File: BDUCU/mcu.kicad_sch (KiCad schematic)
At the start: 15 parts, among them SW1 SW_Push, U8 ATmega328-A, Y1 20MHz

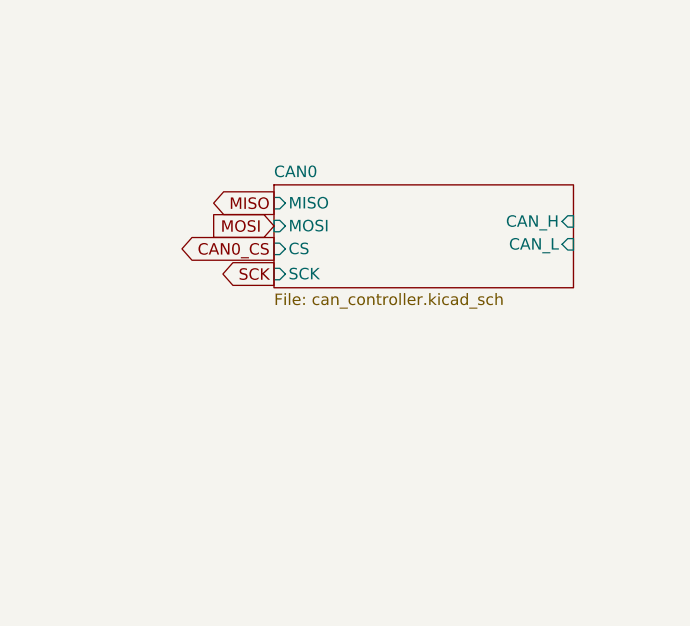
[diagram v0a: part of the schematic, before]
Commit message: BDUCU did stuffs
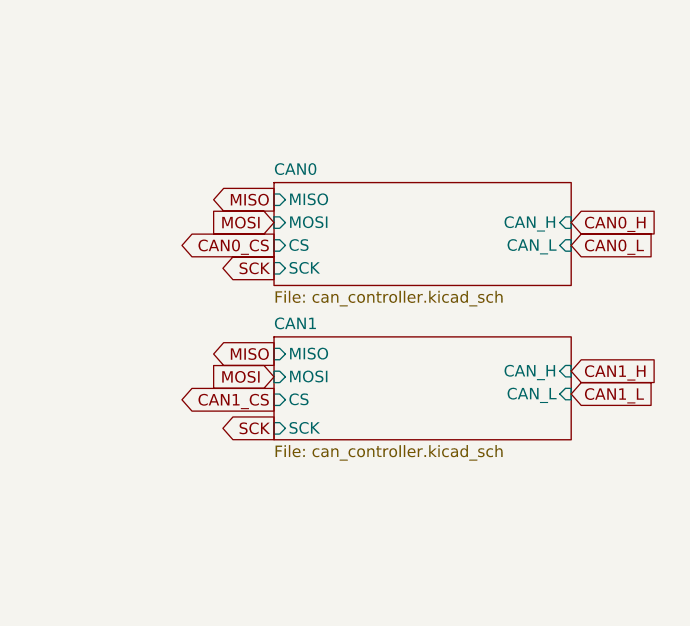
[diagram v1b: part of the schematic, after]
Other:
- added sheet CAN1 (can_controller.kicad_sch)
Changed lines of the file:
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@@
     )
   )
-  (global_label "CAN0_CS" (shape output) (at 209.55 46.736 180) (fields_autoplaced)
-    (effects (font (size 1.27 1.27)) (justify right))
-    (property "Intersheetrefs" "${INTERSHEET_REFS}" (at 198.2191 46.736 0)
+  (global_label "CAN0_CS" (shape output) (at 209.55 46.355 180) (fields_autoplaced)
+    (effects (font (size 1.27 1.27)) (justify right))
+    (property "Intersheetrefs" "${INTERSHEET_REFS}" (at 198.2191 46.355 0)
       (effects (font (size 1.27 1.27)) (justify right) hide)
     )
@@
     )
   )
+  (global_label "CAN0_H" (shape input) (at 242.57 43.815 0) (fields_autoplaced)
+    (effects (font (size 1.27 1.27)) (justify left))
+    (property "Intersheetrefs" "${INTERSHEET_REFS}" (at 252.7519 43.815 0)
+      (effects (font (size 1.27 1.27)) (justify left) hide)
+    )
+  )
+  (global_label "SCK" (shape output) (at 209.55 66.675 180) (fields_autoplaced)
+    (effects (font (size 1.27 1.27)) (justify right))
+    (property "Intersheetrefs" "${INTERSHEET_REFS}" (at 202.8153 66.675 0)
+      (effects (font (size 1.27 1.27)) (justify right) hide)
+    )
+  )
   (global_label "TS_ACT_5" (shape input) (at 71.374 104.648 0) (fields_autoplaced)
     (effects (font (size 1.27 1.27)) (justify left))
@@
     )
   )
+  (global_label "CAN1_CS" (shape output) (at 209.55 63.5 180) (fields_autoplaced)
+    (effects (font (size 1.27 1.27)) (justify right))
+    (property "Intersheetrefs" "${INTERSHEET_REFS}" (at 198.2191 63.5 0)
+      (effects (font (size 1.27 1.27)) (justify right) hide)
+    )
+  )
   (global_label "RST" (shape input) (at 114.935 117.475 180) (fields_autoplaced)
     (effects (font (size 1.27 1.27)) (justify right))
@@
     )
   )
+  (global_label "MOSI" (shape input) (at 209.55 60.96 180) (fields_autoplaced)
+    (effects (font (size 1.27 1.27)) (justify right))
+    (property "Intersheetrefs" "${INTERSHEET_REFS}" (at 202.048 60.96 0)
+      (effects (font (size 1.27 1.27)) (justify right) hide)
+    )
+  )
   (global_label "AIR+_5" (shape output) (at 71.374 94.488 0) (fields_autoplaced)
     (effects (font (size 1.27 1.27)) (justify left))
@@
     )
   )
+  (global_label "MISO" (shape output) (at 209.55 58.42 180) (fields_autoplaced)
+    (effects (font (size 1.27 1.27)) (justify right))
+    (property "Intersheetrefs" "${INTERSHEET_REFS}" (at 201.9686 58.42 0)
+      (effects (font (size 1.27 1.27)) (justify right) hide)
+    )
+  )
   (global_label "HALL_HI" (shape input) (at 71.374 79.248 0) (fields_autoplaced)
     (effects (font (size 1.27 1.27)) (justify left))
@@
     )
   )
+  (global_label "CAN1_H" (shape input) (at 242.57 60.325 0) (fields_autoplaced)
+    (effects (font (size 1.27 1.27)) (justify left))
+    (property "Intersheetrefs" "${INTERSHEET_REFS}" (at 252.7519 60.325 0)
+      (effects (font (size 1.27 1.27)) (justify left) hide)
+    )
+  )
   (global_label "MOSI" (shape input) (at 71.374 56.388 0) (fields_autoplaced)
     (effects (font (size 1.27 1.27)) (justify left))
@@
     )
   )
-  (global_label "MOSI" (shape input) (at 209.55 44.196 180) (fields_autoplaced)
-    (effects (font (size 1.27 1.27)) (justify right))
-    (property "Intersheetrefs" "${INTERSHEET_REFS}" (at 202.048 44.196 0)
+  (global_label "MOSI" (shape input) (at 209.55 43.815 180) (fields_autoplaced)
+    (effects (font (size 1.27 1.27)) (justify right))
+    (property "Intersheetrefs" "${INTERSHEET_REFS}" (at 202.048 43.815 0)
       (effects (font (size 1.27 1.27)) (justify right) hide)
     )
@@
     )
   )
+  (global_label "CAN0_L" (shape input) (at 242.57 46.355 0) (fields_autoplaced)
+    (effects (font (size 1.27 1.27)) (justify left))
+    (property "Intersheetrefs" "${INTERSHEET_REFS}" (at 252.4495 46.355 0)
+      (effects (font (size 1.27 1.27)) (justify left) hide)
+    )
+  )
   (global_label "CAN0_CS" (shape output) (at 71.374 53.848 0) (fields_autoplaced)
     (effects (font (size 1.27 1.27)) (justify left))
@@
     )
   )
-  (global_label "SCK" (shape output) (at 209.55 49.53 180) (fields_autoplaced)
-    (effects (font (size 1.27 1.27)) (justify right))
-    (property "Intersheetrefs" "${INTERSHEET_REFS}" (at 202.8153 49.53 0)
-      (effects (font (size 1.27 1.27)) (justify right) hide)
-    )
-  )
-  (global_label "MISO" (shape output) (at 209.55 41.656 180) (fields_autoplaced)
-    (effects (font (size 1.27 1.27)) (justify right))
-    (property "Intersheetrefs" "${INTERSHEET_REFS}" (at 201.9686 41.656 0)
+  (global_label "SCK" (shape output) (at 209.55 48.895 180) (fields_autoplaced)
+    (effects (font (size 1.27 1.27)) (justify right))
+    (property "Intersheetrefs" "${INTERSHEET_REFS}" (at 202.8153 48.895 0)
+      (effects (font (size 1.27 1.27)) (justify right) hide)
+    )
+  )
+  (global_label "CAN1_L" (shape input) (at 242.57 62.865 0) (fields_autoplaced)
+    (effects (font (size 1.27 1.27)) (justify left))
+    (property "Intersheetrefs" "${INTERSHEET_REFS}" (at 252.4495 62.865 0)
+      (effects (font (size 1.27 1.27)) (justify left) hide)
+    )
+  )
+  (global_label "MISO" (shape output) (at 209.55 41.275 180) (fields_autoplaced)
+    (effects (font (size 1.27 1.27)) (justify right))
+    (property "Intersheetrefs" "${INTERSHEET_REFS}" (at 201.9686 41.275 0)
       (effects (font (size 1.27 1.27)) (justify right) hide)
     )
@@
     )
   )
-  (sheet (at 209.55 39.624) (size 33.274 11.43) (fields_autoplaced)
+  (sheet (at 209.55 39.37) (size 33.02 11.43) (fields_autoplaced)
     (stroke (width 0.1524) (type solid))
     (fill (color 0 0 0 0.0000))
-    (property "Sheetname" "CAN0" (at 209.55 38.9124 0)
+    (property "Sheetname" "CAN0" (at 209.55 38.6584 0)
       (effects (font (size 1.27 1.27)) (justify left bottom))
     )
-    (property "Sheetfile" "can_controller.kicad_sch" (at 209.55 51.6386 0)
+    (property "Sheetfile" "can_controller.kicad_sch" (at 209.55 51.3846 0)
       (effects (font (size 1.27 1.27)) (justify left top))
     )
-    (pin "MISO" input (at 209.55 41.656 180)
+    (pin "MISO" input (at 209.55 41.275 180)
       (effects (font (size 1.27 1.27)) (justify left))
     )
-    (pin "MOSI" input (at 209.55 44.196 180)
+    (pin "MOSI" input (at 209.55 43.815 180)
       (effects (font (size 1.27 1.27)) (justify left))
     )
-    (pin "CS" input (at 209.55 46.736 180)
+    (pin "CS" input (at 209.55 46.355 180)
       (effects (font (size 1.27 1.27)) (justify left))
     )
-    (pin "SCK" input (at 209.55 49.53 180)
+    (pin "SCK" input (at 209.55 48.895 180)
       (effects (font (size 1.27 1.27)) (justify left))
     )
-    (pin "CAN_H" input (at 242.824 43.688 0)
-      (effects (font (size 1.27 1.27)) (justify right))
-    )
-    (pin "CAN_L" input (at 242.824 46.228 0)
+    (pin "CAN_H" input (at 242.57 43.815 0)
+      (effects (font (size 1.27 1.27)) (justify right))
+    )
+    (pin "CAN_L" input (at 242.57 46.355 0)
       (effects (font (size 1.27 1.27)) (justify right))
     )
@@
       )
     )
+  )
+  (sheet (at 209.55 56.515) (size 33.02 11.43) (fields_autoplaced)
+    (stroke (width 0.1524) (type solid))
+    (fill (color 0 0 0 0.0000))
+    (property "Sheetname" "CAN1" (at 209.55 55.8034 0)
+      (effects (font (size 1.27 1.27)) (justify left bottom))
+    )
+    (property "Sheetfile" "can_controller.kicad_sch" (at 209.55 68.5296 0)
+      (effects (font (size 1.27 1.27)) (justify left top))
+    )
+    (pin "MISO" input (at 209.55 58.42 180)
+      (effects (font (size 1.27 1.27)) (justify left))
+    )
+    (pin "MOSI" input (at 209.55 60.96 180)
+      (effects (font (size 1.27 1.27)) (justify left))
+    )
+    (pin "CS" input (at 209.55 63.5 180)
+      (effects (font (size 1.27 1.27)) (justify left))
+    )
+    (pin "SCK" input (at 209.55 66.675 180)
+      (effects (font (size 1.27 1.27)) (justify left))
+    )
+    (pin "CAN_H" input (at 242.57 60.325 0)
+      (effects (font (size 1.27 1.27)) (justify right))
+    )
+    (pin "CAN_L" input (at 242.57 62.865 0)
+      (effects (font (size 1.27 1.27)) (justify right))
+    )
+    (instances
+      (project "BDUCU"
+        (path "/9942a424-e19d-4ffb-8473-f960b5c811cf/8fc427df-2d97-44b9-b479-5014f2f05880" (page "12"))
+      )
+    )

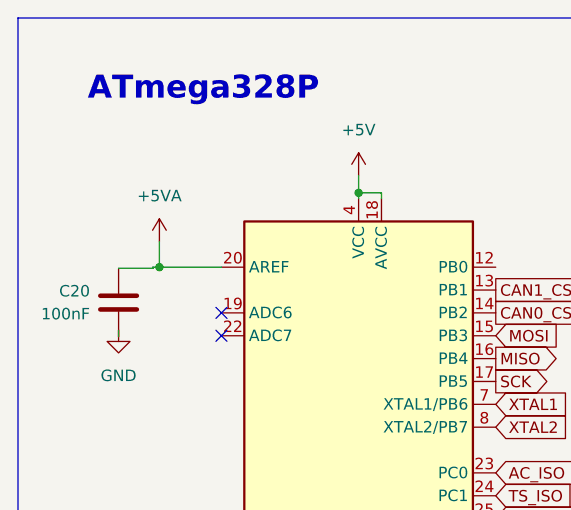
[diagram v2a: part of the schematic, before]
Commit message: BDUCU COMMIT
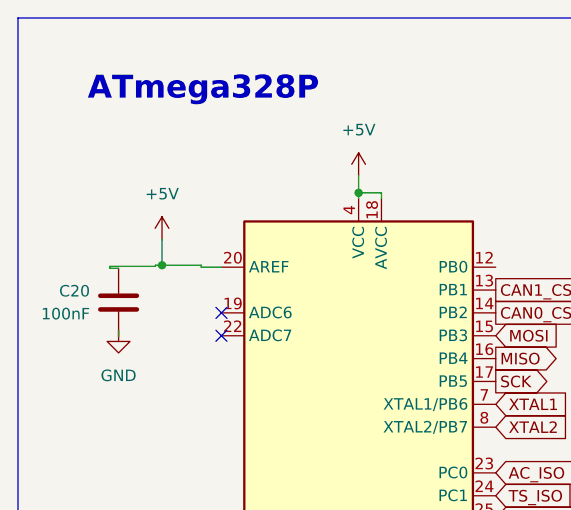
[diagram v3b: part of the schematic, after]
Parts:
- AVR-ISP1: footprint Connector_PinHeader_2.54mm:PinHeader_2x03_P2.54mm_Vertical -> Connector_PinHeader_2.54mm:PinHeader_2x03_P2.54mm_Vertical_SMD
- Y1: value 20MHz -> 16MHz
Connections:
- net +5VA is gone; now on net +5V: C20.2, U8.20 (AREF)
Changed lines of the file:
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@@
 	)
 	(junction
-		(at 34.001 48.768)
+		(at 34.29 48.5525)
 		(diameter 0)
 		(color 0 0 0 0)
@@
 	(wire
 		(pts
-			(xy 34.001 48.768) (xy 40.894 48.768)
+			(xy 28.483 48.6795) (xy 33.563 48.6795)
+		)
+		(stroke
+			(width 0)
+			(type default)
+		)
+	)
+	(wire
+		(pts
+			(xy 34.29 48.5525) (xy 38.643 48.5525)
 		)
 		(stroke
@@
 	(wire
 		(pts
-			(xy 34.001 45.9355) (xy 34.001 48.768)
+			(xy 34.29 45.72) (xy 34.29 48.5525)
+		)
+		(stroke
+			(width 0)
+			(type default)
+		)
+	)
+	(wire
+		(pts
+			(xy 28.483 48.895) (xy 29.464 48.895)
 		)
 		(stroke
@@
 	(wire
 		(pts
+			(xy 28.483 48.6795) (xy 28.483 48.895)
+		)
+		(stroke
+			(width 0)
+			(type default)
+		)
+	)
+	(wire
+		(pts
 			(xy 111.76 86.995) (xy 111.76 95.25)
 		)
@@
 	(wire
 		(pts
-			(xy 33.274 48.895) (xy 33.274 48.768)
+			(xy 33.563 48.6795) (xy 33.563 48.5525)
 		)
 		(stroke
@@
 	(wire
 		(pts
+			(xy 38.643 48.768) (xy 40.894 48.768)
+		)
+		(stroke
+			(width 0)
+			(type default)
+		)
+	)
+	(wire
+		(pts
 			(xy 100.965 41.275) (xy 100.965 40.64)
 		)
@@
 	(wire
 		(pts
+			(xy 38.643 48.5525) (xy 38.643 48.768)
+		)
+		(stroke
+			(width 0)
+			(type default)
+		)
+	)
+	(wire
+		(pts
 			(xy 125.73 86.995) (xy 125.73 95.25)
 		)
@@
 	(wire
 		(pts
-			(xy 33.274 48.768) (xy 34.001 48.768)
-		)
-		(stroke
-			(width 0)
-			(type default)
-		)
-	)
-	(wire
-		(pts
-			(xy 29.464 48.895) (xy 33.274 48.895)
+			(xy 33.563 48.5525) (xy 34.29 48.5525)
 		)
 		(stroke
@@
 				(path "/9942a424-e19d-4ffb-8473-f960b5c811cf/8fc427df-2d97-44b9-b479-5014f2f05880"
 					(reference "D3")
+					(unit 1)
+				)
+			)
+		)
+	)
+	(symbol
+		(lib_id "power:+5V")
+		(at 34.29 45.72 0)
+		(unit 1)
+		(exclude_from_sim no)
+		(in_bom yes)
+		(on_board yes)
+		(dnp no)
+		(fields_autoplaced yes)
+		(property "Reference" "#PWR033"
+			(at 34.29 49.53 0)
+			(effects
+				(font
+					(size 1.27 1.27)
+				)
+				(hide yes)
+			)
+		)
+		(property "Value" "+5V"
+			(at 34.29 40.64 0)
+			(effects
+				(font
+					(size 1.27 1.27)
+				)
+			)
+		)
+		(property "Footprint" ""
+			(at 34.29 45.72 0)
+			(effects
+				(font
+					(size 1.27 1.27)
+				)
+				(hide yes)
+			)
+		)
+		(property "Datasheet" ""
+			(at 34.29 45.72 0)
+			(effects
+				(font
+					(size 1.27 1.27)
+				)
+				(hide yes)
+			)
+		)
+		(property "Description" ""
+			(at 34.29 45.72 0)
+			(effects
+				(font
+					(size 1.27 1.27)
+				)
+			)
+		)
+		(pin "1"
+		)
+		(instances
+			(project "BDUCU"
+				(path "/9942a424-e19d-4ffb-8473-f960b5c811cf/8fc427df-2d97-44b9-b479-5014f2f05880"
+					(reference "#PWR033")
 					(unit 1)
 				)
@@
 			)
 		)
-		(property "Footprint" "Connector_PinHeader_2.54mm:PinHeader_2x03_P2.54mm_Vertical"
+		(property "Footprint" "Connector_PinHeader_2.54mm:PinHeader_2x03_P2.54mm_Vertical_SMD"
 			(at 120.015 114.935 0)
 			(effects
@@
 	)
 	(symbol
-		(lib_id "power:+5VA")
-		(at 34.001 45.9355 0)
-		(unit 1)
-		(exclude_from_sim no)
-		(in_bom yes)
-		(on_board yes)
-		(dnp no)
-		(fields_autoplaced yes)
-		(property "Reference" "#PWR035"
-			(at 34.001 49.7455 0)
-			(effects
-				(font
-					(size 1.27 1.27)
-				)
-				(hide yes)
-			)
-		)
-		(property "Value" "+5VA"
-			(at 34.001 40.8555 0)
-			(effects
-				(font
-					(size 1.27 1.27)
-				)
-			)
-		)
-		(property "Footprint" ""
-			(at 34.001 45.9355 0)
-			(effects
-				(font
-					(size 1.27 1.27)
-				)
-				(hide yes)
-			)
-		)
-		(property "Datasheet" ""
-			(at 34.001 45.9355 0)
-			(effects
-				(font
-					(size 1.27 1.27)
-				)
-				(hide yes)
-			)
-		)
-		(property "Description" ""
-			(at 34.001 45.9355 0)
-			(effects
-				(font
-					(size 1.27 1.27)
-				)
-			)
-		)
-		(pin "1"
-		)
-		(instances
-			(project "BDUCU"
-				(path "/9942a424-e19d-4ffb-8473-f960b5c811cf/8fc427df-2d97-44b9-b479-5014f2f05880"
-					(reference "#PWR035")
-					(unit 1)
-				)
-			)
-		)
-	)
-	(symbol
 		(lib_id "Device:C")
 		(at 100.965 36.83 180)
@@
 			)
 		)
-		(property "Value" "20MHz"
+		(property "Value" "16MHz"
 			(at 104.775 64.008 90)
 			(effects
@@
 		(exclude_from_sim no)
 		(in_bom yes)
-		(on_board no)
+		(on_board yes)
 		(dnp no)
 		(property "Reference" "C20"

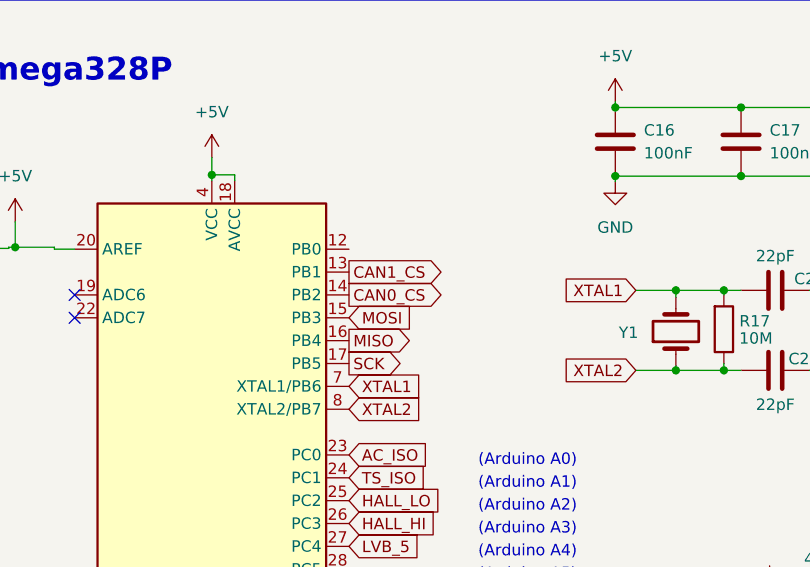
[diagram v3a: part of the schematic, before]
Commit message: BDUCU finalised
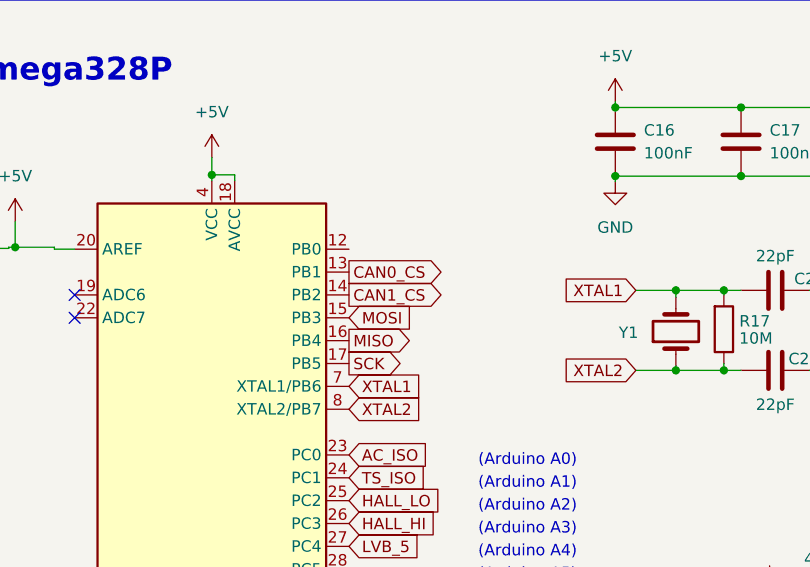
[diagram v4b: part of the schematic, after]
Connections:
- net CAN0_CS: now also U8.13 (PB1); no longer U8.14 (PB2)
- net CAN1_CS: now also U8.14 (PB2); no longer U8.13 (PB1)
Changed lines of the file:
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@@
 	(global_label "CAN0_CS"
 		(shape output)
-		(at 71.374 53.848 0)
+		(at 71.374 51.308 0)
 		(fields_autoplaced yes)
 		(effects
@@
 		)
 		(property "Intersheetrefs" "${INTERSHEET_REFS}"
-			(at 82.7049 53.848 0)
+			(at 82.7049 51.308 0)
 			(effects
 				(font
@@
 	(global_label "CAN1_CS"
 		(shape output)
-		(at 71.374 51.308 0)
+		(at 71.374 53.848 0)
 		(fields_autoplaced yes)
 		(effects
@@
 		)
 		(property "Intersheetrefs" "${INTERSHEET_REFS}"
-			(at 82.7049 51.308 0)
+			(at 82.7049 53.848 0)
 			(effects
 				(font
